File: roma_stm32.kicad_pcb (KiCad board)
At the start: 4 copper layers, 62.5 x 72 mm, 38 parts, among them J1 CAN, J2 Power, J3 Debug_Port, J4 GPIO, J5 IO_I2C, J6 IO_SPI, J7 IO_UART, SW1 SW_RST, U1 TJA1051T-3, U2 STM32L432KBU6, U3 ADP1108AR-3.3, U4 ADP1108AR-5

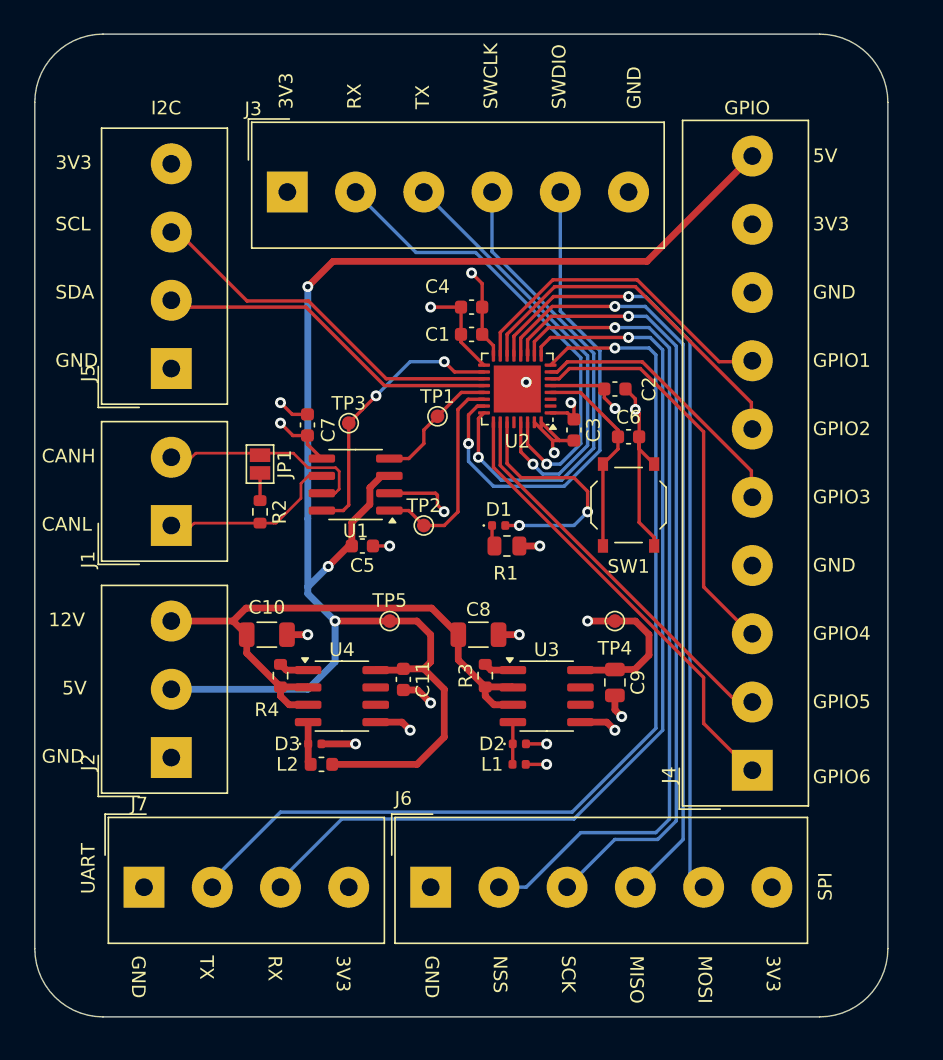
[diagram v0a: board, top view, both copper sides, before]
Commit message: Fix PCB
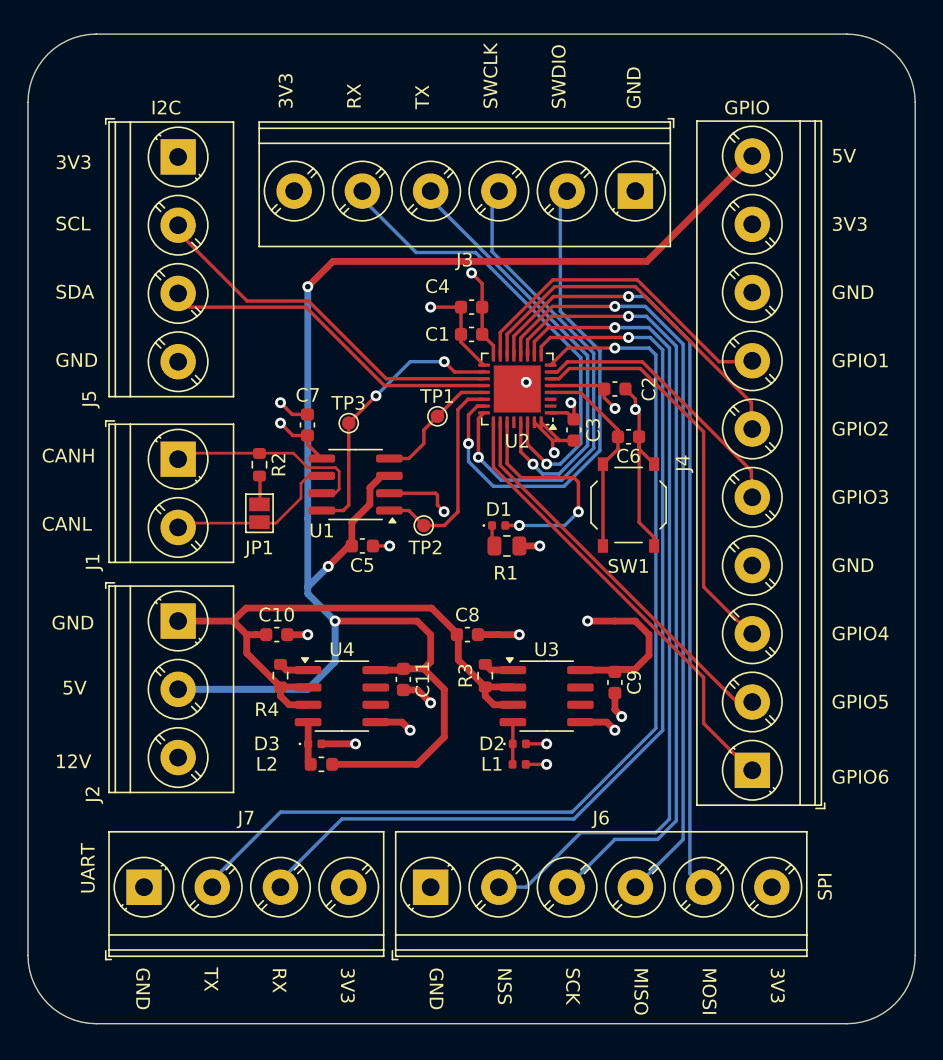
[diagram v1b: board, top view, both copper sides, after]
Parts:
- removed TP4, TP5: TestPoint, TestPoint:TestPoint_Pad_D1.0mm
- C10, C8: footprint Capacitor_SMD:C_1206_3216Metric -> Capacitor_SMD:C_0603_1608Metric
- C9: footprint Capacitor_SMD:C_0805_2012Metric -> Capacitor_SMD:C_0603_1608Metric
- J1: footprint TerminalBlock_Altech:Altech_AK100_1x02_P5.00mm -> TerminalBlock_Phoenix:TerminalBlock_Phoenix_PT-1,5-2-5.0-H_1x02_P5.00mm_Horizontal
- J2: footprint TerminalBlock_Altech:Altech_AK100_1x03_P5.00mm -> TerminalBlock_Phoenix:TerminalBlock_Phoenix_PT-1,5-3-5.0-H_1x03_P5.00mm_Horizontal
- J3: footprint TerminalBlock_Altech:Altech_AK100_1x06_P5.00mm -> TerminalBlock_Phoenix:TerminalBlock_Phoenix_PT-1,5-6-5.0-H_1x06_P5.00mm_Horizontal
- J4: footprint TerminalBlock_Altech:Altech_AK100_1x10_P5.00mm -> TerminalBlock_Phoenix:TerminalBlock_Phoenix_PT-1,5-10-5.0-H_1x10_P5.00mm_Horizontal
- J5: value IO_I2C -> I2C; footprint TerminalBlock_Altech:Altech_AK100_1x04_P5.00mm -> TerminalBlock_Phoenix:TerminalBlock_Phoenix_PT-1,5-4-5.0-H_1x04_P5.00mm_Horizontal
- J6: value IO_SPI -> SPI; footprint TerminalBlock_Altech:Altech_AK100_1x06_P5.00mm -> TerminalBlock_Phoenix:TerminalBlock_Phoenix_PT-1,5-6-5.0-H_1x06_P5.00mm_Horizontal
- J7: value IO_UART -> UART; footprint TerminalBlock_Altech:Altech_AK100_1x04_P5.00mm -> TerminalBlock_Phoenix:TerminalBlock_Phoenix_PT-1,5-4-5.0-H_1x04_P5.00mm_Horizontal
- JP1: value CAN_Resistor -> SolderJumper_2_Open
- R1: value 3.3K -> 120R
- U2: value STM32L432KBU6 -> STM32L432KBUx
- moved J3 25.5 mm to (199.5, 46.5), turned to 180 degrees
- moved J5 15.5 mm to (166.0, 44.0), turned to -90 degrees
- moved J2 10.0 mm to (166.0, 78.0), turned to -90 degrees
- moved J1 4.88 mm to (166.0, 66.1), turned to -90 degrees
- moved JP1 3.60 mm to (172.0, 70.1), turned to 90 degrees
- moved R2 3.45 mm to (172.0, 66.5)
- moved C8 0.80 mm to (187.2, 79.0)
- moved C10 0.73 mm to (173.2, 79.0)
- turned C6 to 180 degrees
- turned C7 to -90 degrees
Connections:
- C6 pad 1: Net-(U2-NRST) -> GND
- C6 pad 2: GND -> Net-(U2-NRST)
- C7 pad 1: +3V3 -> GND
- C7 pad 2: GND -> +3V3
- J1 pad 1: CAN- -> CAN_H
- J1 pad 2: CAN+ -> CAN_L
- J2 pad 1: GND -> +12V
- J2 pad 3: +12V -> GND
- J3 pad 2: Debug_UART_RX -> JTAG_SWDIO
- J3 pad 3: Debug_UART_TX -> JTAG_SWCLK
- J3 pad 4: JTAG_SWCLK -> Debug_UART_TX
- J3 pad 5: JTAG_SWDIO -> Debug_UART_RX
- J5 pad 2: IO_I2C_SDA -> IO_I2C_SCL
- J5 pad 3: IO_I2C_SCL -> IO_I2C_SDA
- JP1 pad 1: CAN+ -> CAN_L
- R2 pad 1: Net-(JP1-B) -> CAN_H
- R2 pad 2: CAN- -> Net-(JP1-B)
- U1 pad 6: CAN- -> CAN_L
- U1 pad 7: CAN+ -> CAN_H
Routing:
- net CAN_H: track 0.00 -> 15.6 mm
- net CAN+: track 15.6 -> 0.00 mm
- net CAN_L: track 0.00 -> 13.1 mm
- net CAN-: track 13.1 -> 0.00 mm
- net GND: track 55.1 -> 56.6 mm
- net +12V: track 43.1 -> 44.6 mm
- net LED: track 17.7 -> 16.8 mm
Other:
- board size 62.5 x 72 mm -> 65 x 72.5 mm
